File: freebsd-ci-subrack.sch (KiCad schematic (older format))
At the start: 25 parts

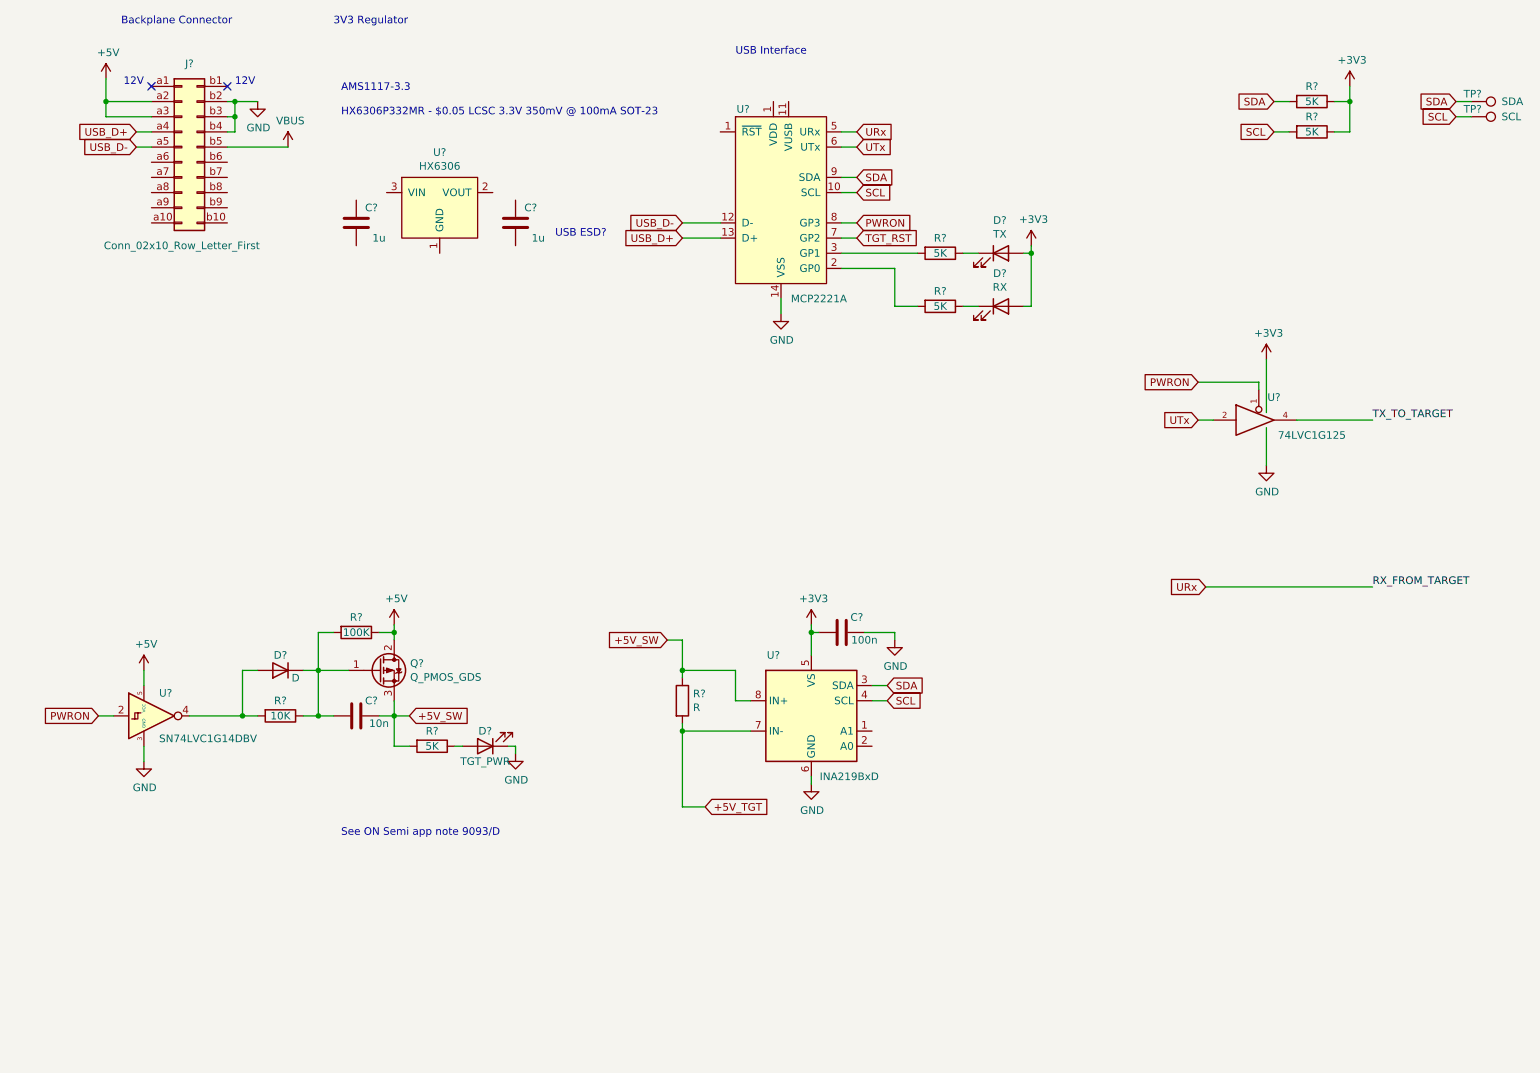
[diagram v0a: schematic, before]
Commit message: Snapshot after choosing most parts
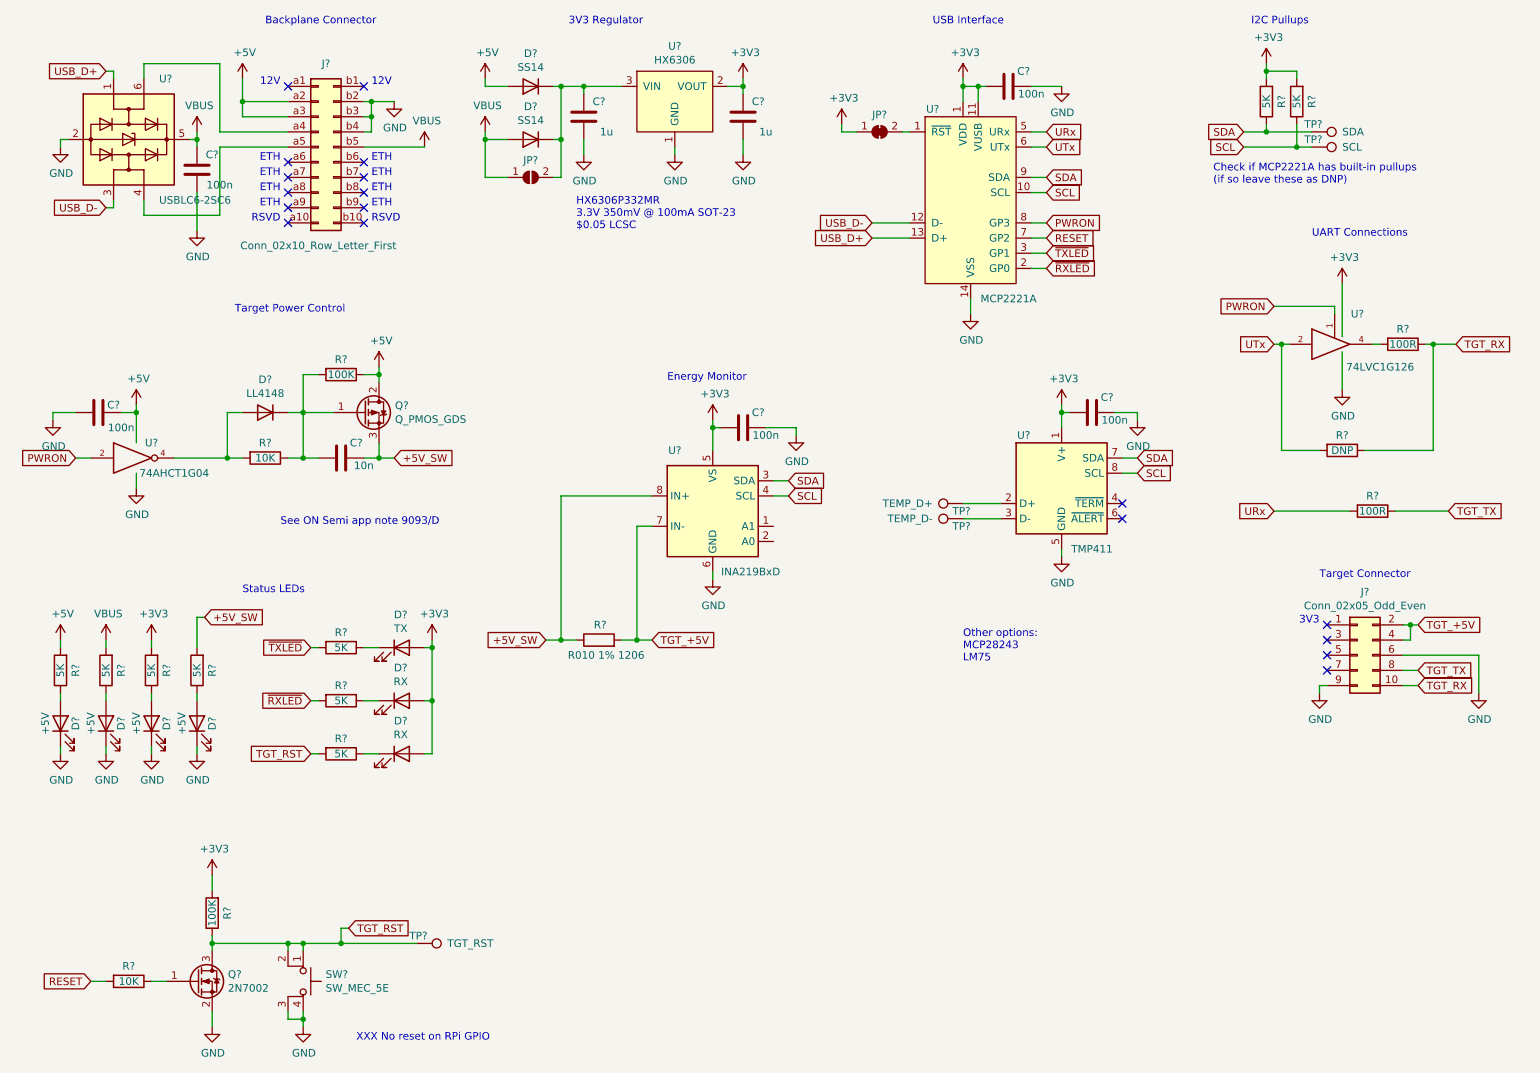
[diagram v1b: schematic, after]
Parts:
- removed D?: TGT_PWR, symbol Device:LED
- removed D?: D, symbol Device:D
- removed R? (x4): 5K, symbol Device:R
- removed R?: 100K, symbol Device:R
- removed R?: 10K, symbol Device:R
- removed U?: 74LVC1G125, symbol 74xGxx:74LVC1G125
- removed U?: SN74LVC1G14DBV, Package_TO_SOT_SMD:SOT-23-5, symbol 74xGxx:SN74LVC1G14DBV
- added C? (x4): 100n, symbol Device:C
- added D? (x4): +5V, symbol Device:LED
- added D? (x2): SS14, Diode_SMD:D_SMA, symbol Device:D
- added D?: LL4148, Diode_SMD:D_MiniMELF, symbol Diode:LL4148
- added D?: RX, symbol Device:LED
- added J?: Conn_02x05_Odd_Even, symbol Connector_Generic:Conn_02x05_Odd_Even
- added JP?: SolderJumper_2_Open, symbol Jumper:SolderJumper_2_Open
- added JP?: SolderJumper_2_Bridged, symbol Jumper:SolderJumper_2_Bridged
- added Q?: 2N7002, Package_TO_SOT_SMD:SOT-23, symbol Transistor_FET:2N7002
- added R?: 100K, symbol Device:R
- added R?: 10K, symbol Device:R
- added R? (x8): 5K, Resistor_SMD:R_0603_1608Metric, symbol Device:R
- added R? (x2): 100R, Resistor_SMD:R_0603_1608Metric, symbol Device:R
- added R?: 100K, Resistor_SMD:R_0603_1608Metric, symbol Device:R
- added R?: 10K, Resistor_SMD:R_0603_1608Metric, symbol Device:R
- added R?: DNP, Resistor_SMD:R_0603_1608Metric, symbol Device:R
- added SW?: SW_MEC_5E, symbol Switch:SW_MEC_5E
- added TP?: TGT_RST, symbol Connector:TestPoint
- added TP?: TEMP_D+, symbol Connector:TestPoint
- added TP?: TEMP_D-, symbol Connector:TestPoint
- added U?: USBLC6-2SC6, Package_TO_SOT_SMD:SOT-23-6, symbol Power_Protection:USBLC6-2SC6
- added U?: 74AHCT1G04, symbol 74xGxx:74AHCT1G04
- added U?: 74LVC1G126, symbol 74xGxx:74LVC1G126
- added U?: TMP411, symbol Sensor_Temperature:TMP411
- R?: value R -> R010 1% 1206; footprint (none) -> Resistor_SMD:R_1206_3216Metric
- R?: footprint (none) -> Resistor_SMD:R_0603_1608Metric
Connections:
- net +5V is gone; now on net +3V3: J?.a2 (Pin_a2), J?.a3 (Pin_a3), Q?.2 (D)
- net +3V3: now also C?.2, U?.1 (~RST), U?.11 (VUSB), U?.2 (VOUT), C?.1, C?.2, C?.2, D?.2 (A), D?.2 (A), JP?.1 (A), R?.1, R?.2, R?.2, R?.2, R?.2, R?.2, U?.1 (V+), U?.5 (VCC), U?.5 (VCC)
- net +5V_SW: now also R?.2
- net GND: now also C?.1, C?.1, U?.1 (GND), C?.1, C?.1, C?.1, C?.2, D?.1 (K), D?.1 (K), D?.1 (K), D?.1 (K), J?.6 (Pin_6), J?.9 (Pin_9), Q?.2 (S), SW?.3 (K), SW?.4 (A), U?.2 (GND), U?.3 (GND), U?.3 (GND), U?.5 (GND)
- net PWRON: now also U?.1, U?.2
- net SCL: now also R?.1, U?.8 (SCL)
- net SDA: now also R?.1, U?.7 (SDA)
- net TGT_RST: now also Q?.3 (D), R?.1, R?.2, SW?.1, SW?.2, TP?.1; no longer U?.7 (GP2)
- net URx: now also R?.2
- net USB_D+: now also U?.1 (I/O1); no longer J?.a4 (Pin_a4)
- net USB_D-: now also U?.3 (I/O2); no longer J?.a5 (Pin_a5)
- net UTx: now also R?.2, U?.2
- net VBUS: now also C?.2, D?.2 (A), JP?.1 (A), R?.2, U?.5 (VBUS)
- net ~RXLED: now reaches U?.2 (GP0)
- net ~RXLED: now also R?.2
- net ~TXLED: now reaches R?.2, U?.3 (GP1)
- net at D?.1 (K): now also R?.1
- net at U?.3 (VIN): now also C?.2, D?.1 (K), D?.1 (K), JP?.2 (B)
- net at C?.2, Q?.1 (G): now also D?.1 (K), R?.1, R?.2
- net +5V_TGT renamed TGT_+5V
- net TGT_+5V: now also J?.2 (Pin_2), J?.4 (Pin_4)
- new net: J?.a4 (Pin_a4), U?.6 (I/O1)
- new net: J?.a5 (Pin_a5), U?.4 (I/O2)
- new net: JP?.2 (B), U?.1 (~RST)
- new net: Q?.1 (G), R?.1
- new net: D?.2 (A), R?.2, U?.4
- new net: D?.2 (A), R?.1 (x4)
- new net: R?.2, U?.4
- new net: D?.1 (K), R?.1
- new net: TP?.1, U?.2 (D+)
- new net: TP?.1, U?.3 (D-)
- new net RESET: R?.2, U?.7 (GP2)
- new net TGT_RX: J?.10 (Pin_10), R?.1, R?.1
- new net TGT_TX: J?.8 (Pin_8), R?.1
- no-connect marks 2 -> 18
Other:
- note added: "3V3"
- note added: "Check if MCP2221A has built-in pullups\n(if so leave these as DNP)"
- note added: "ETH"
- note added: "Energy Monitor"
- note added: "HX6306P332MR\n3.3V 350mV @ 100mA SOT-23\n$0.05 LCSC \n"
- note added: "I2C Pullups"
- note added: "Other options:\nMCP28243\nLM75"
- note added: "RSVD"
- note added: "Status LEDs"
- note added: "Target Connector"
- note added: "Target Power Control"
- note added: "UART Connections"
- note added: "XXX No reset on RPi GPIO"
- note removed: "AMS1117-3.3\n\nHX6306P332MR - $0.05 LCSC 3.3V 350mV @ 100mA SOT-23"
- note removed: "USB ESD?"
- moved on the sheet: C?, D?, J?, Q?, R?, TP?, U?
